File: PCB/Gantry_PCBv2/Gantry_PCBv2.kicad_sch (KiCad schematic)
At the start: 138 parts, among them J1 Screw_Terminal_01x02, J10 B2B-XH-A_LF__SN_, J11 USB_C_Receptacle_USB2.0_16P, J12 Conn_01x04_Pin, J13 Conn_01x04_Pin, J14 Conn_01x04_Pin, J15 Conn_01x04_Pin, J2 DCJ200-10-A-XX-X_REVA, J3 Conn_01x03_Pin, J4 Conn_01x14, J5 B2B-XH-A_LF__SN_, J6 B2B-XH-A_LF__SN_, J7 B2B-XH-A_LF__SN_, J8 Conn_01x14, J9 Conn_01x10, Q1 NMOS, Q2 SS8050, Q3 SS8050, SW1 SW_0, SW2 SW_EN, U1 ESP32-WROOM-32E, U10 74HC245, U11 74HC245, U2 MP1584, U3 CH340C, U4 TLV75733PDBV, U5 DRV8825_STEPPER_MOTOR_DRIVER_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, U6 DRV8825_STEPPER_MOTOR_DRIVER_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, U7 TB6612FNG H-bridge Motor Driv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, U8 DRV8825_STEPPER_MOTOR_DRIVER_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, U9 DRV8825_STEPPER_MOTOR_DRIVER_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

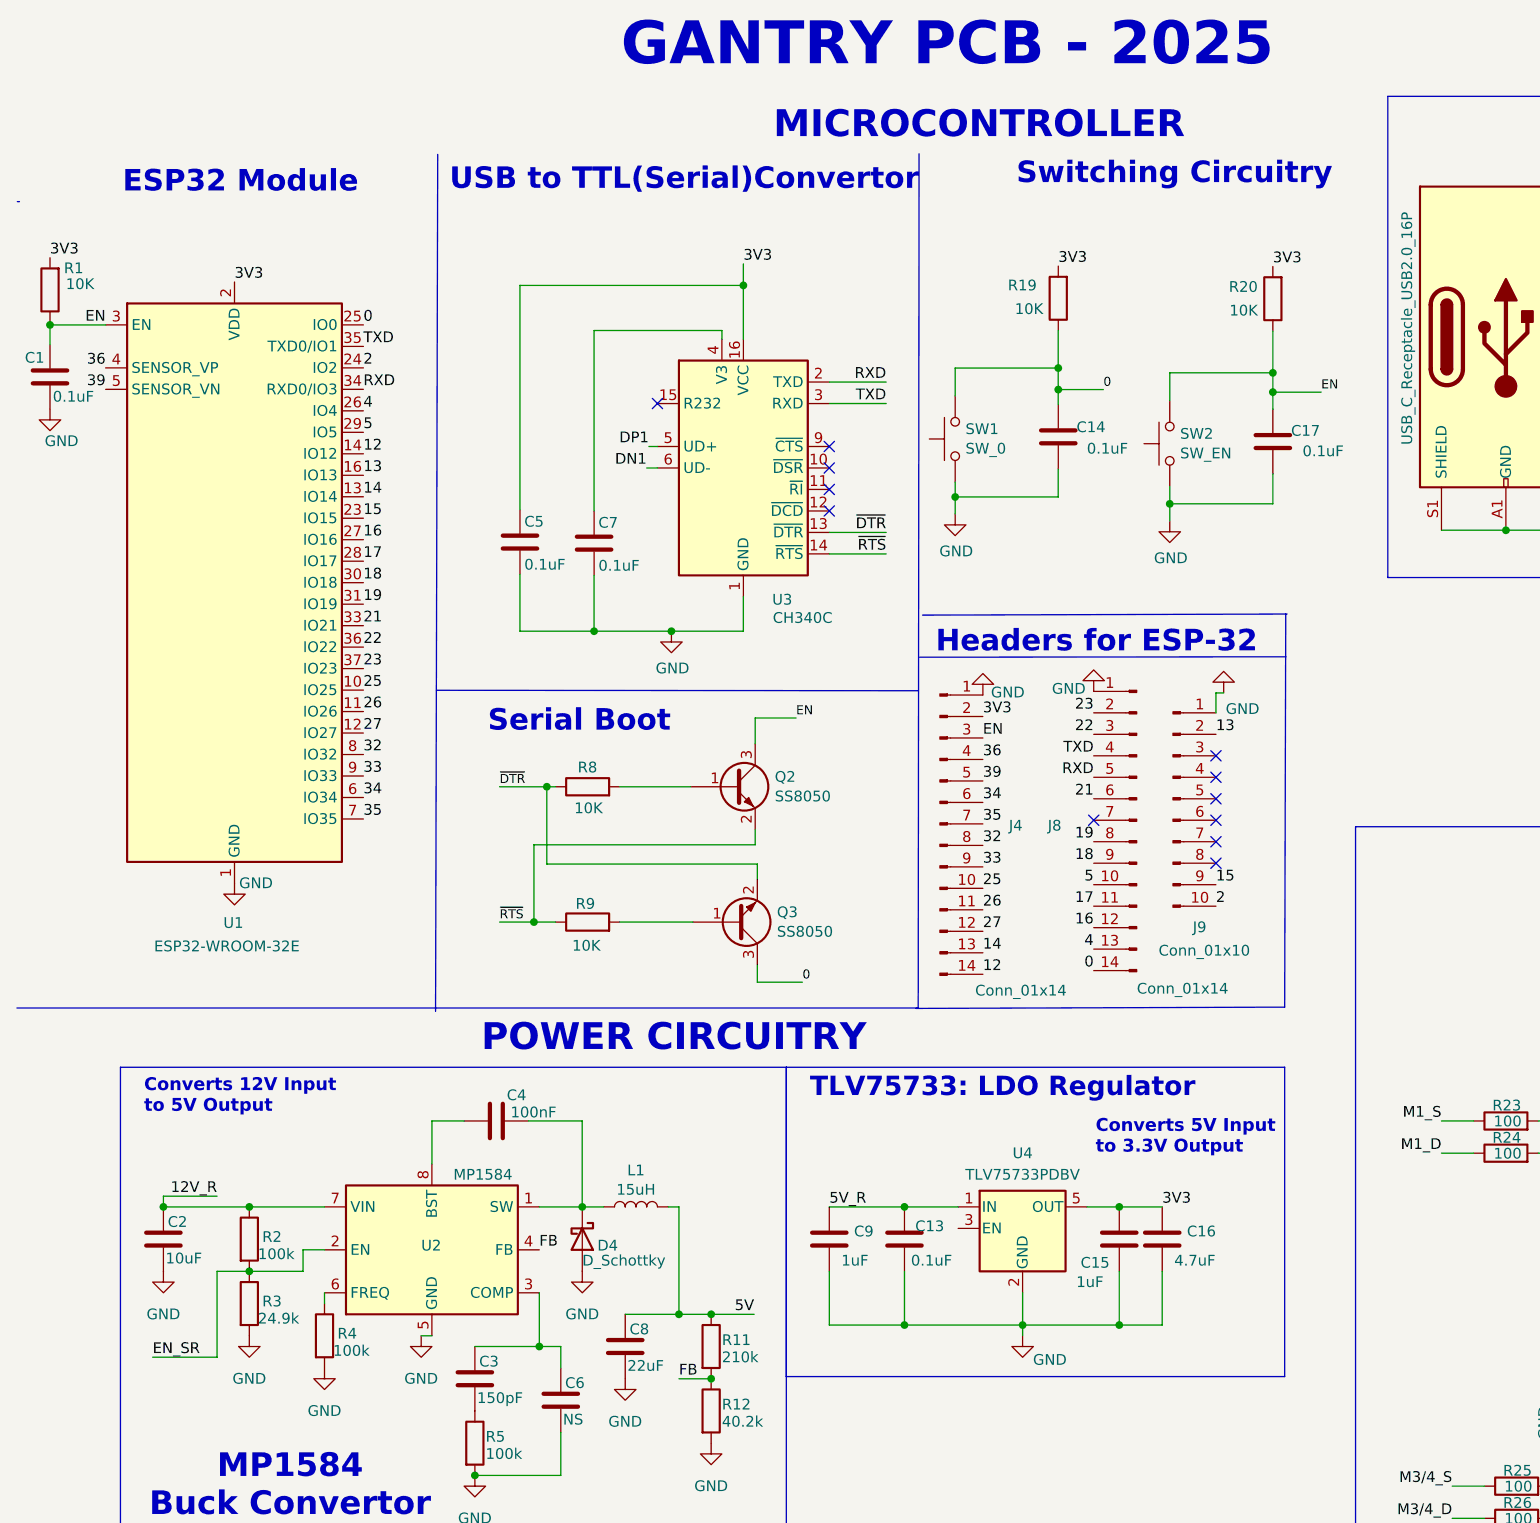
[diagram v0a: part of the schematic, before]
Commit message: Added Footprints and Formatting
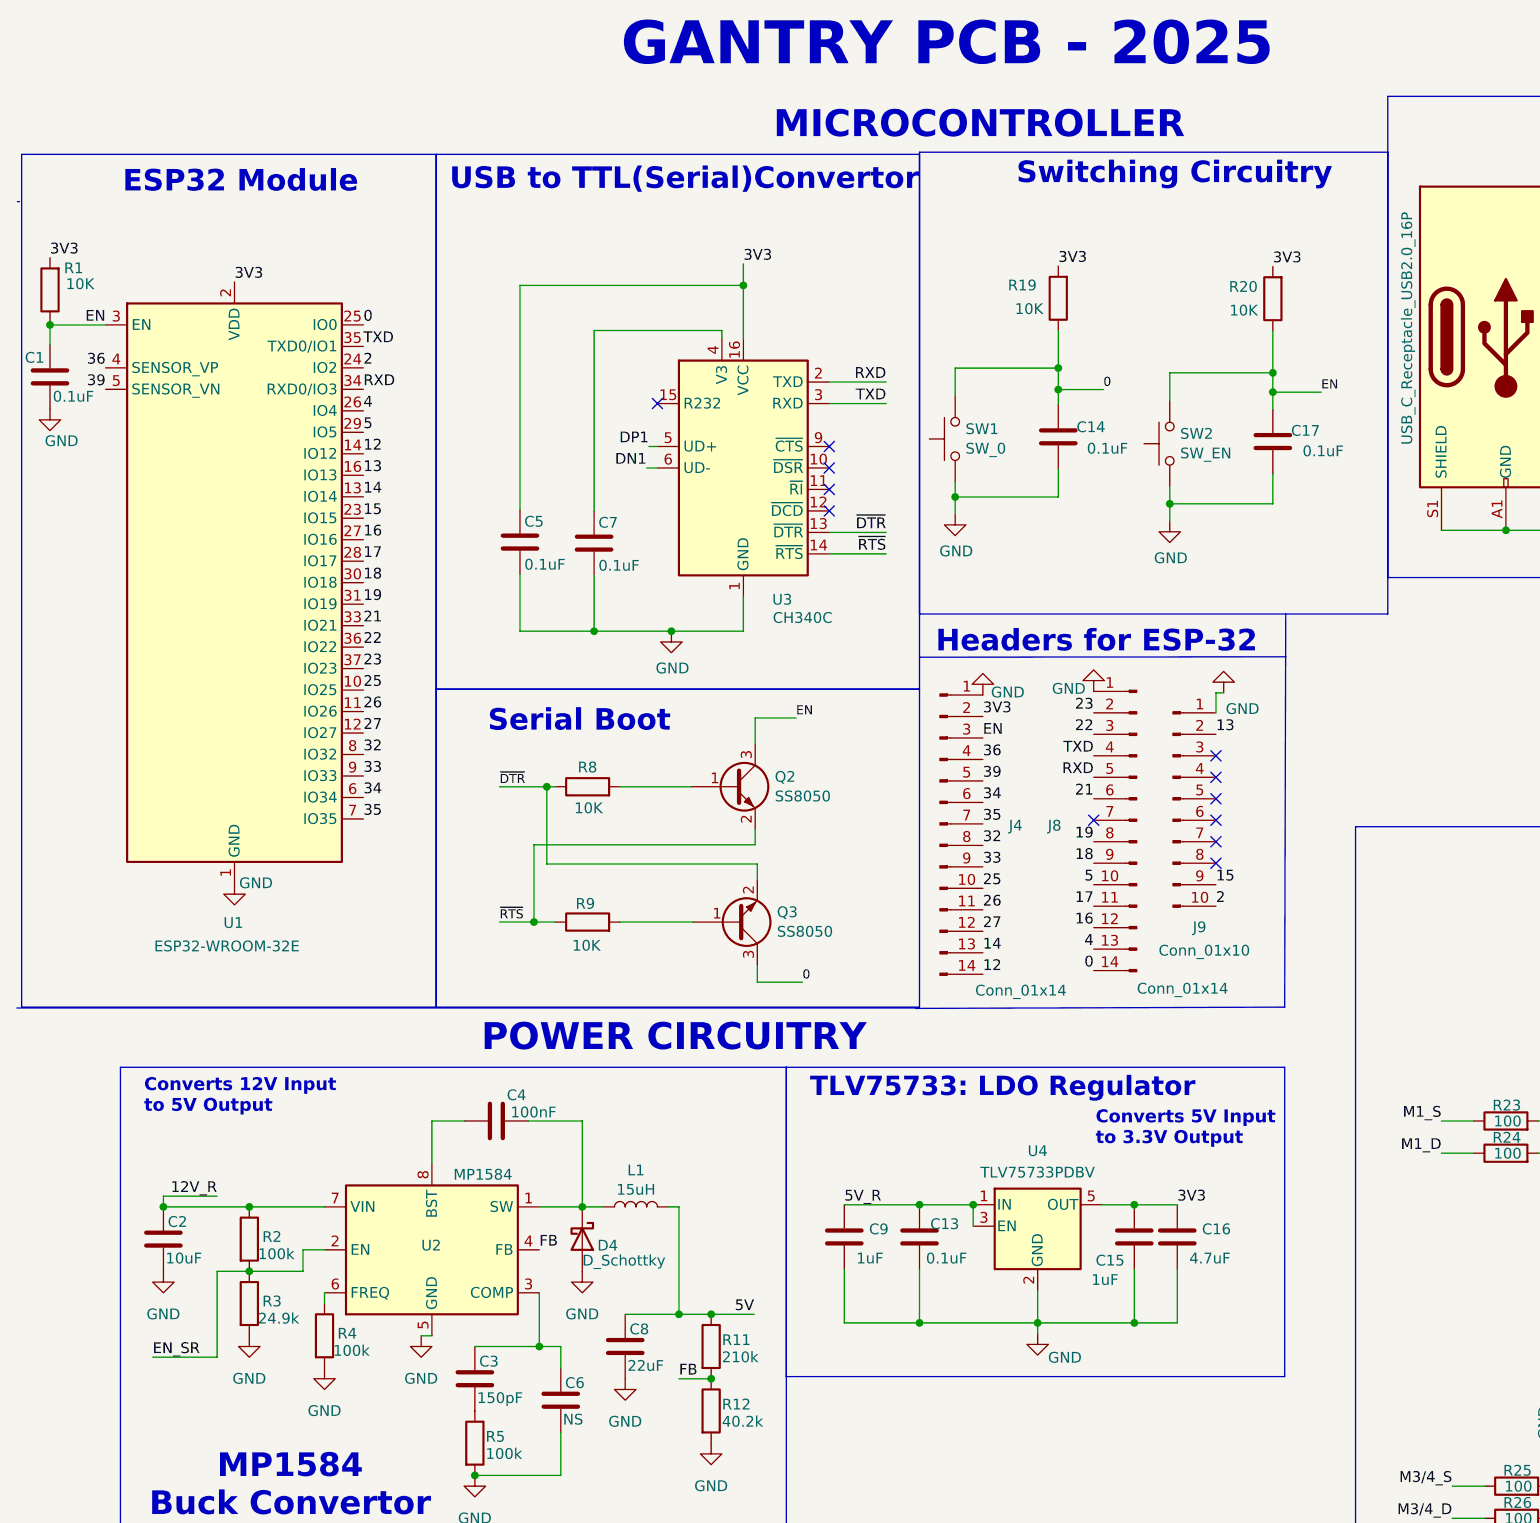
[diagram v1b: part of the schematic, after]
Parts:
- F3: footprint (none) -> Fuse:Fuse_Littelfuse-LVR100
- Q1: footprint (none) -> Package_TO_SOT_THT:TO-247-3_Vertical
- U10, U11: footprint (none) -> Package_SO:SOIC-20W_7.5x15.4mm_P1.27mm
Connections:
- net 5V_R: now also U4.3 (EN)
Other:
- moved on the sheet: C13, C15, C16, C9, U4
